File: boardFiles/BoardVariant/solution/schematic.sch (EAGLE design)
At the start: 40 parts, among them IC1 MSP430F1491, IC3 CP2102, U1 TPS62122_DRV_6

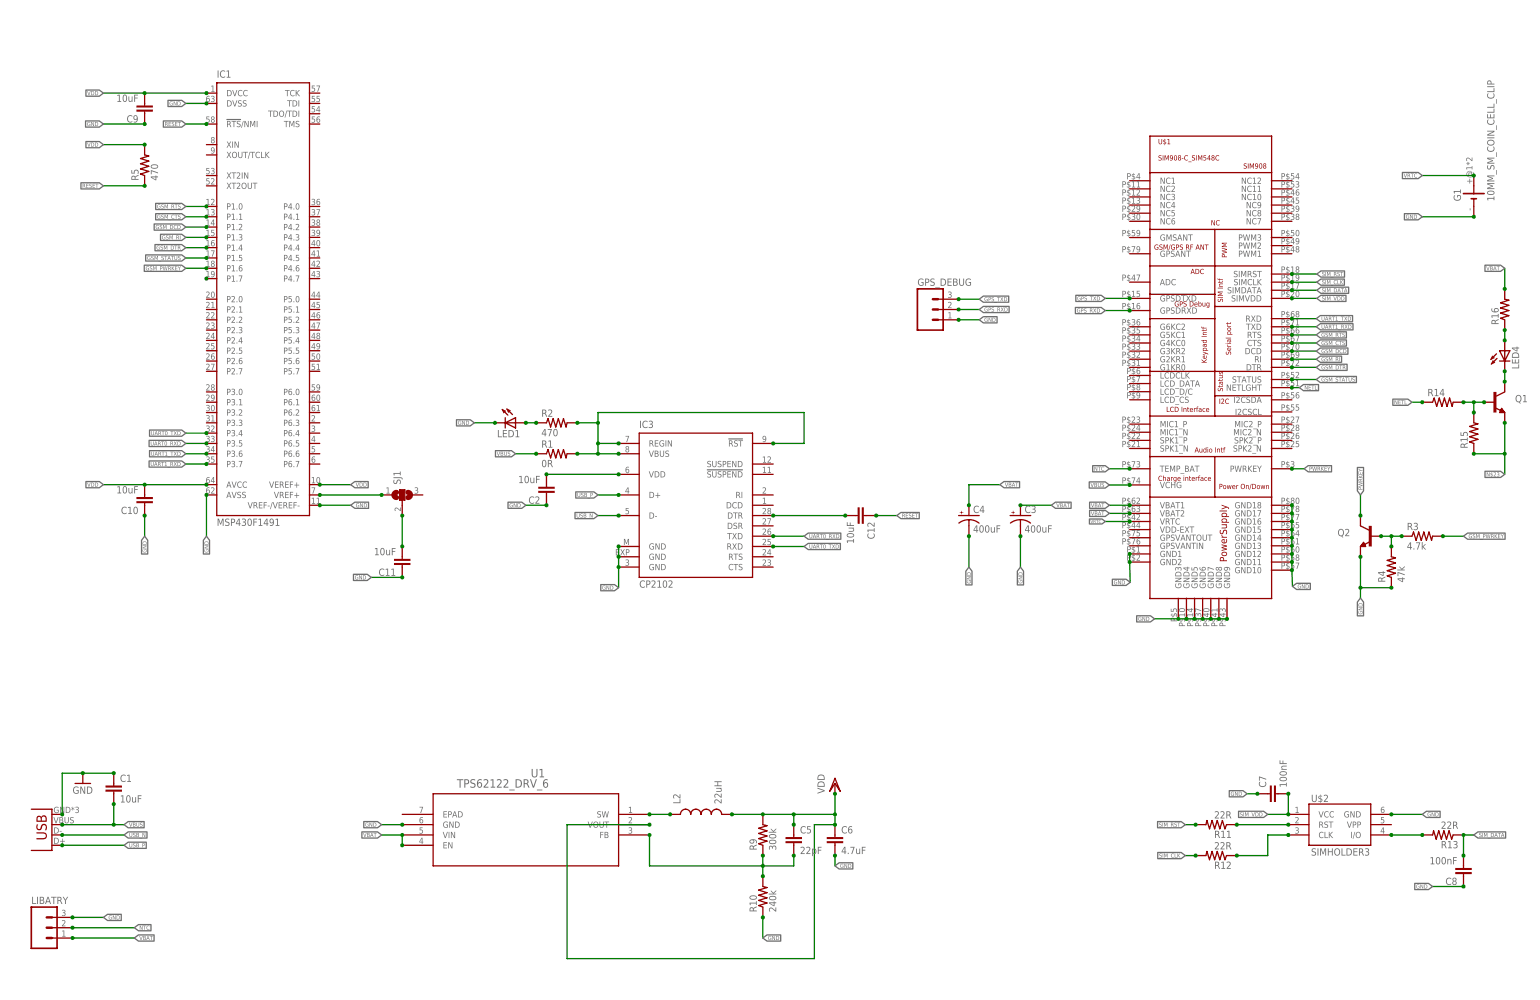
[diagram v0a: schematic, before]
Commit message: normal Push.
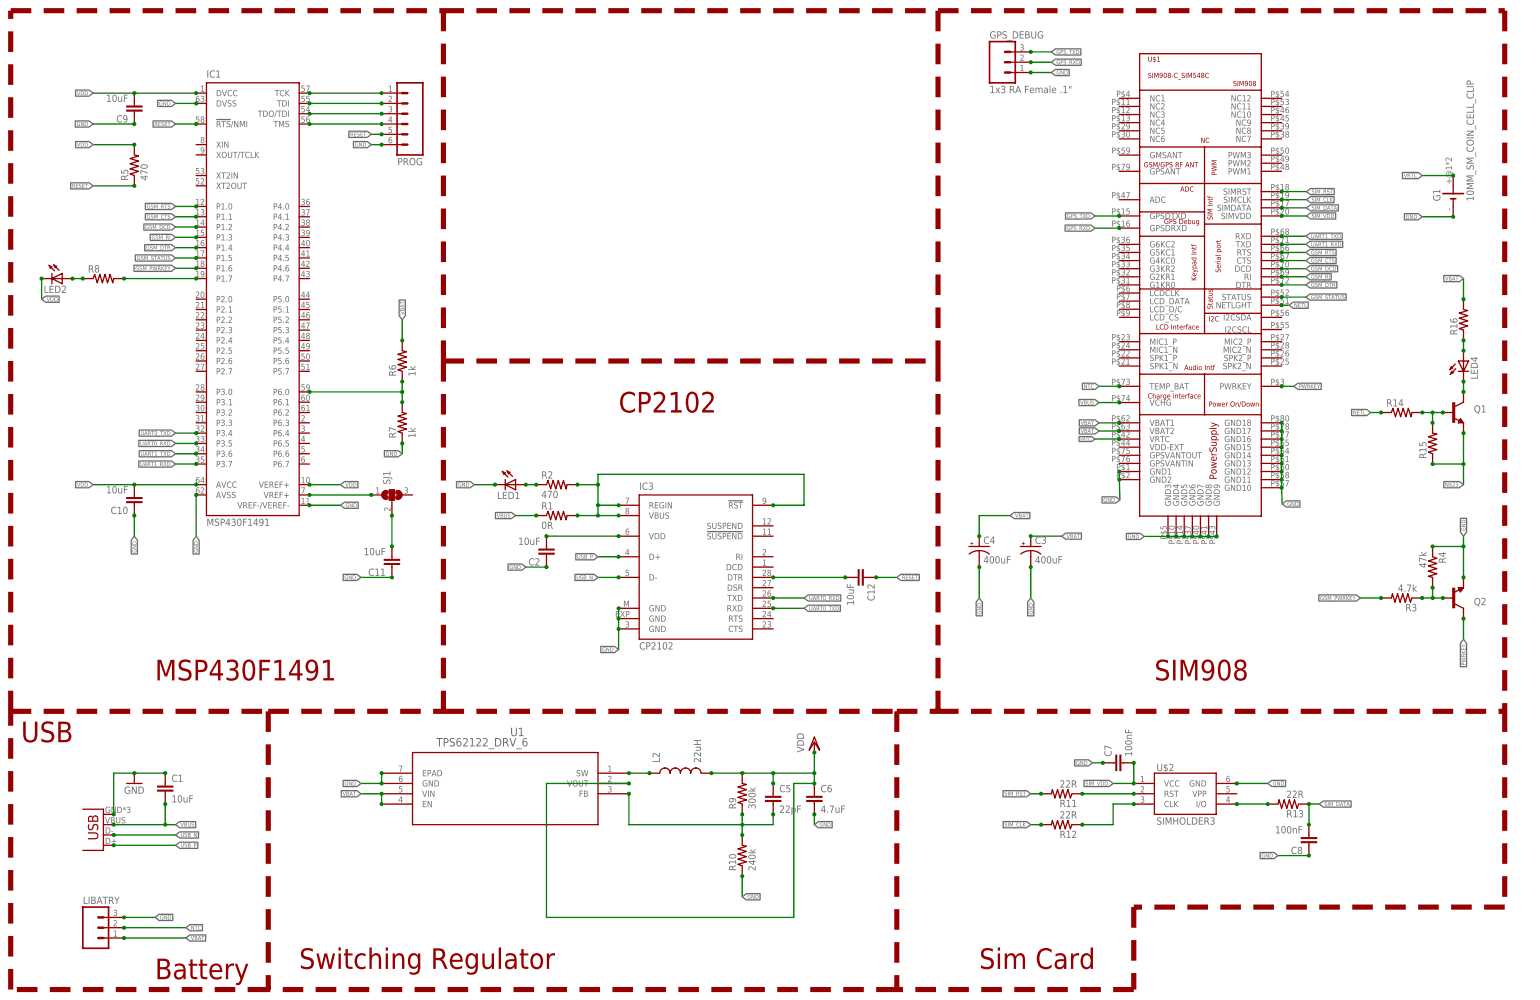
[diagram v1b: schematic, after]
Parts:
- added LED2: (no value), led:LEDSML0603
- added PROG: (no value), SparkFun-Connectors:M06SMD-STRAIGHT
- added R6, R7: 1k, SparkFun-Passives:RESISTOR0402-RES
- added R8: (no value), SparkFun:RESISTOR0402-RES
- GPS_DEBUG: value (none) -> 1x3 RA Female .1"; device SparkFun-Connectors:M03PTH -> SparkFun-Connectors:M03SMD_RA_FEMALE
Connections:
- new net N$1: IC1.TCK, PROG.1
- new net N$13: LED2.A, R8.1
- new net N$20: IC1.P6.0, R6.1, R7.2
- new net N$3: IC1.TDI, PROG.2
- new net N$6: IC1.TDO/TDI, PROG.3
- new net N$9: IC1.TMS, PROG.4
- net GND: now also PROG.6, R7.1, U1.EPAD
- net N$25: now also R8.2
- net RESET: now also PROG.5
- net VBAT: now also R6.2
- net VDD: now also LED2.C
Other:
- note added: "Battery"
- note added: "CP2102"
- note added: "MSP430F1491"
- note added: "SIM908"
- note added: "Sim Card"
- note added: "Switching Regulator"
- note added: "USB"
- moved on the sheet: C1, C10, C11, C12, C2, C3, C4, C5, C6, C7, C8, C9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
